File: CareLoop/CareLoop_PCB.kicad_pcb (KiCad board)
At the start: 6 copper layers, 38.5 x 22.3 mm, 73 parts, among them J1 Conn_Coaxial_Small, J1_Battery1 Conn_01x02_Pin, J1_DEBUG1 Conn_01x04_Pin, J2 USB_B_Micro, U1 MCP1700x-180xxMB, U2 MAX30102, U3 MPU-6050, U4 MCP1700x-330xxMB, U5 TP4056-42-ESOP8, U6 nRF52840-QFXX, U7 PCA9306, Y1 32MHz, Y2 32.768kHz

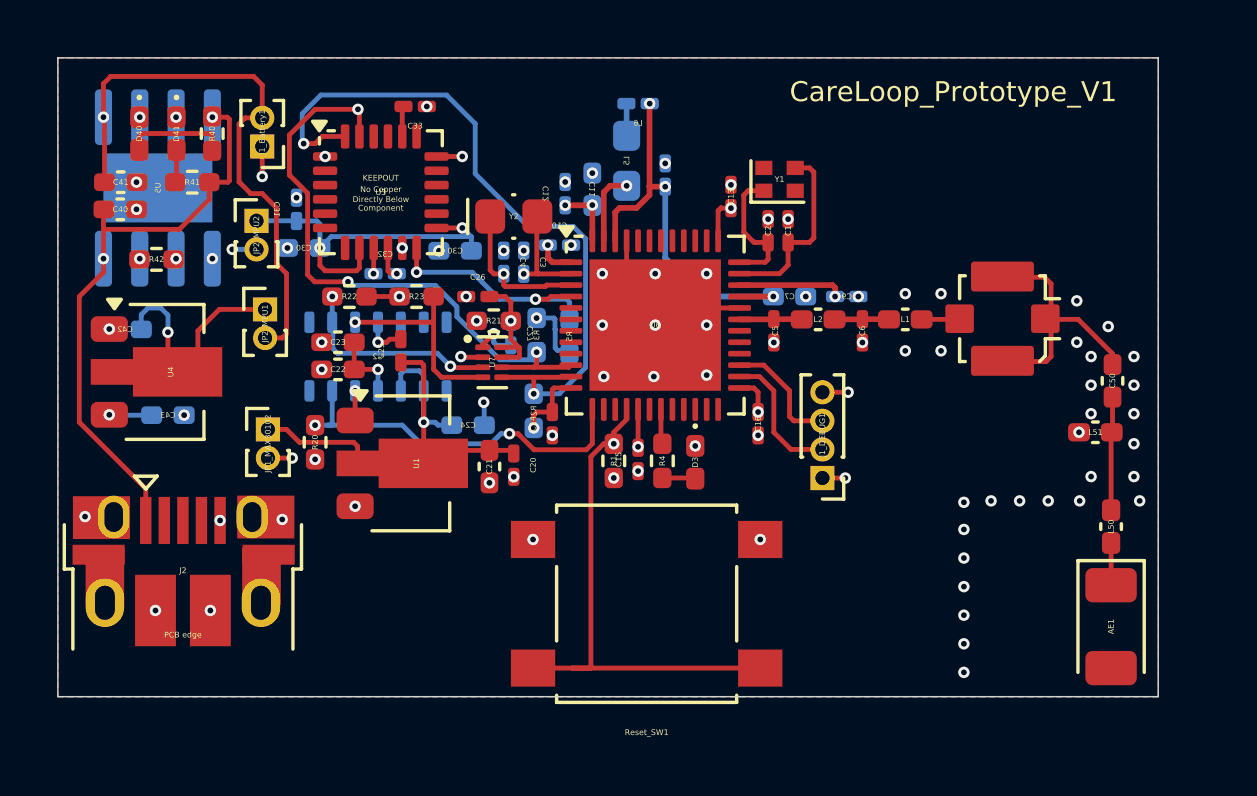
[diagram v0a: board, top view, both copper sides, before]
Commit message: PCB update
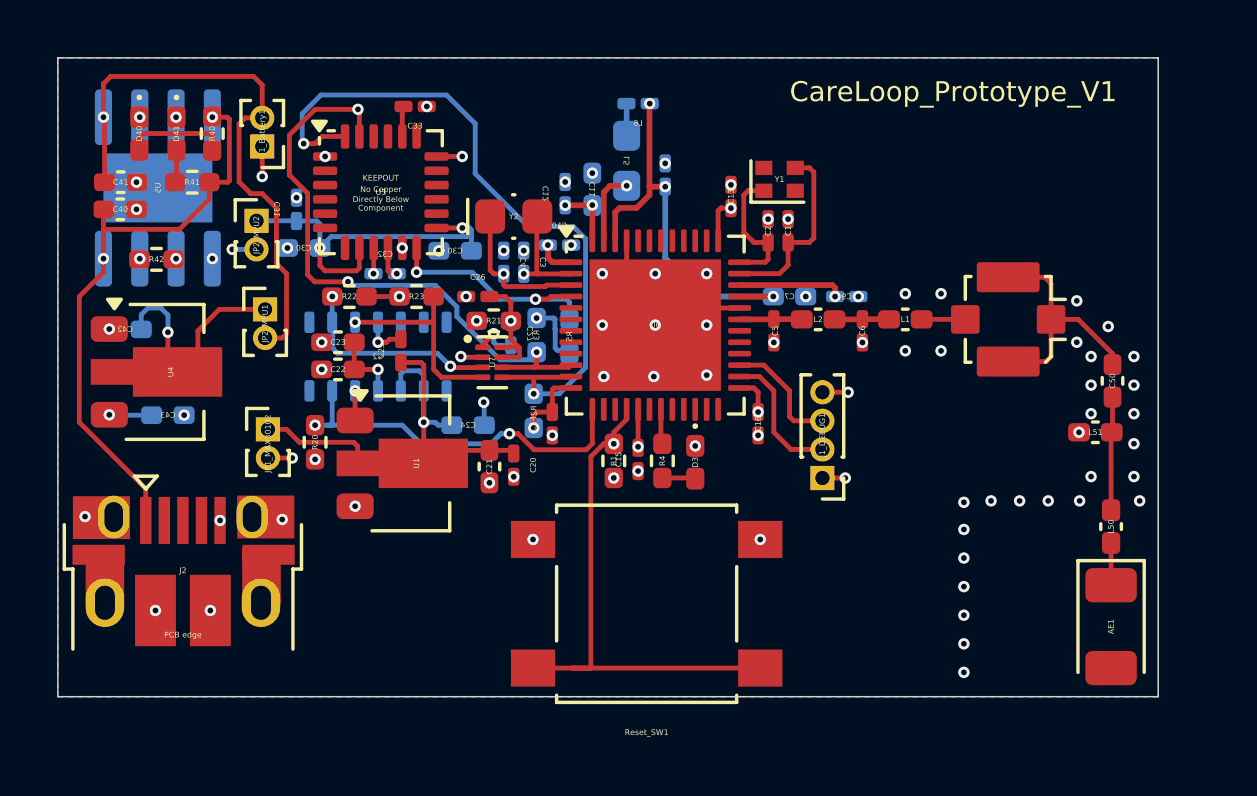
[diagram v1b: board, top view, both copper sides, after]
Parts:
- moved J1 0.20 mm to (158.6, 96.2)
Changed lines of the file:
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@@
 	(footprint "Connector_Coaxial:U.FL_Molex_MCRF_73412-0110_Vertical"
 		(layer "F.Cu")
-		(at 158.4 96.125 -90)
+		(at 158.6 96.15 -90)
 		(descr "Molex Microcoaxial RF Connectors (MCRF), mates Hirose U.FL, (http://www.molex.com/pdm_docs/sd/734120110_sd.pdf)")
 		(tags "mcrf hirose ufl u.fl microcoaxial")
@@
 	)
 	(segment
-		(start 139.8175 93.2675)
-		(end 139.5 92.95)
-		(width 0.17)
-		(layer "B.Cu")
-		(net 77)
-	)
-	(segment
 		(start 139.8175 93.75)
 		(end 139.8175 93.2675)
@@
 	)
 	(segment
+		(start 139.75 92.95)
+		(end 139.5 92.95)
+		(width 0.17)
+		(layer "B.Cu")
+		(net 77)
+	)
+	(segment
 		(start 134.5175 92.8175)
 		(end 134.5175 93.65)
@@
 		(width 0.17)
 		(layer "B.Cu")
+		(net 77)
+	)
+	(segment
+		(start 139.8175 93.2675)
+		(end 139.8175 93.0175)
+		(width 0.17)
+		(layer "B.Cu")
+		(net 77)
+	)
+	(segment
+		(start 139.8175 93.0175)
+		(end 139.75 92.95)
+		(width 0.17)
+		(layer "B.Cu")
